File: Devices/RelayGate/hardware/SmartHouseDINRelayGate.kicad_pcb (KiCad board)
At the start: 2 copper layers, 31 x 82 mm, 14 parts, among them P1 CONN_UPDOWN_ONOFF_PWR_GND, P2 CONN_IN_DOWN_UP, Q1 Q_NPN_EBC, Q2 Q_NPN_EBC, Q3 Q_NPN_BCE_DTC124, Q4 Q_NPN_BCE_DTC124, U2 RELAY_1C, U3 RELAY_1C

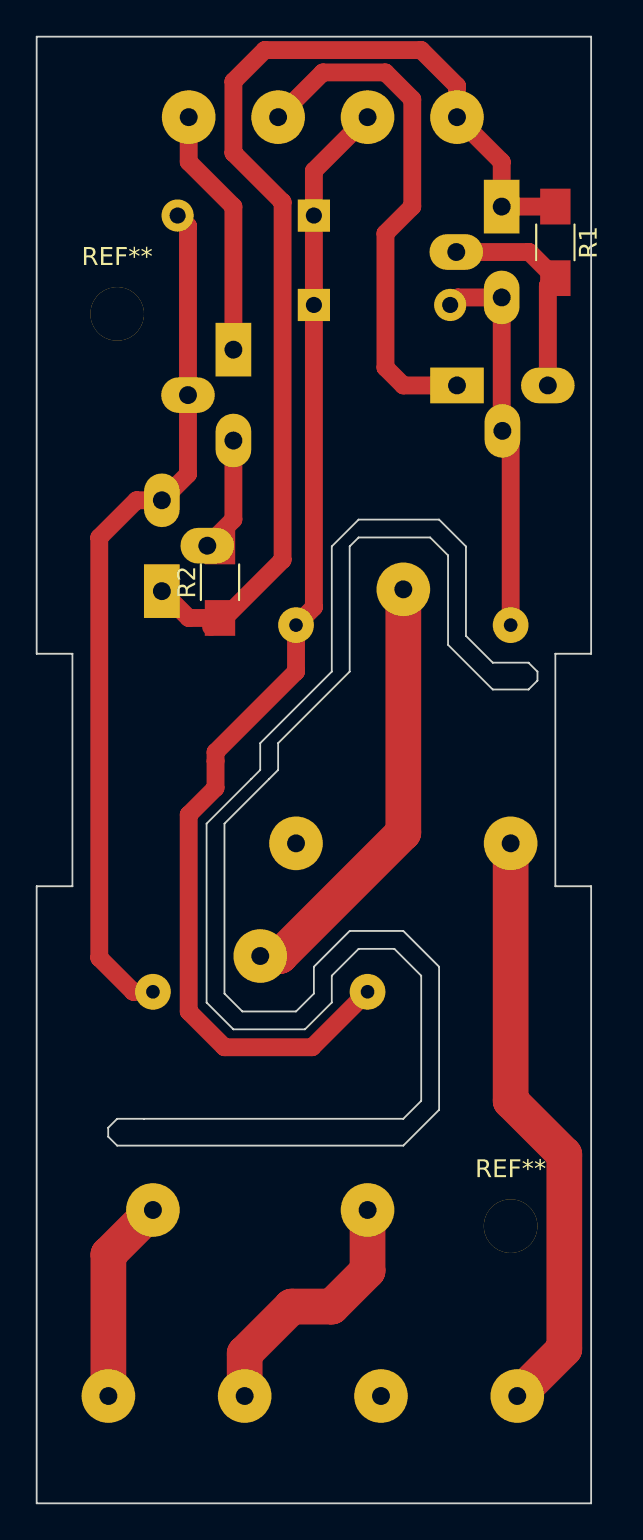
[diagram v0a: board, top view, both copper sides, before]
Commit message: -Devices updates
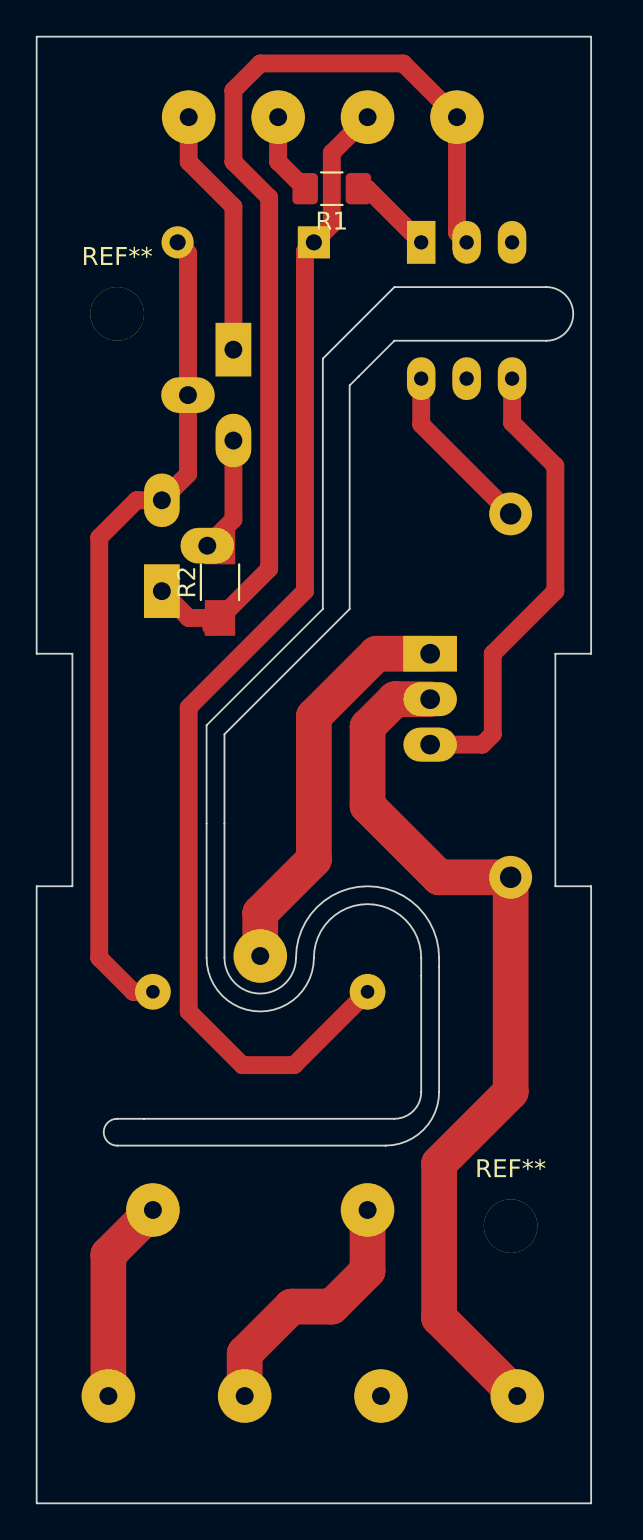
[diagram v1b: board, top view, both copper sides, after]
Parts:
- removed D1: D, Diodes_ThroughHole:D_A-405_P7.62mm_Horizontal
- removed Q3: Q_NPN_BCE_DTC124, TO_SOT_Packages_THT:TO-92_Rugged
- removed U2: RELAY_1C, SmartHouseLib:RELAY_TRU_1C
- added R3: R, Resistor_THT:R_Axial_DIN0414_L11.9mm_D4.5mm_P20.32mm_Horizontal, B.Cu at (275.0, 97.5)
- added U1: MOC3020M, Package_DIP:DIP-6_W7.62mm_LongPads, B.Cu at (270.0, 62.0)
- Q1: value Q_NPN_EBC -> BTA16-600B; footprint TO_SOT_Packages_THT:TO-92_Rugged -> Package_TO_SOT_THT:TO-220-3_Vertical
- R1: value R4K7 -> R; footprint Resistors_SMD:R_1206_HandSoldering -> Resistor_SMD:R_1206_3216Metric_Pad1.42x1.75mm_HandSolder
- moved Q1 25.3 mm to (270.5, 85.0)
- moved R1 12.9 mm to (265.0, 59.0), turned to 180 degrees
- moved D2 1.50 mm to (264.0, 62.0)
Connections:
- Q1 pad 1: Net-(P1-Pad4) -> Net-(Q1-Pad1)
- Q1 pad 2: Net-(Q1-Pad2) -> Net-(P2-Pad4)
- R1 pad 1: Net-(P1-Pad4) -> Net-(R1-Pad1)
- R1 pad 2: Net-(Q1-Pad2) -> Net-(P1-Pad2)
- U3 pad 3: Net-(U2-Pad3) -> Net-(Q1-Pad1)
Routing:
- net Net-(P1-Pad2): track 29.2 -> 4.63 mm
- net Net-(U2-Pad3): track 24.5 -> 0.00 mm
- net Net-(Q1-Pad1): track 0.00 -> 22.6 mm
- net Net-(P2-Pad4): track 33.2 -> 50.7 mm
- net Net-(Q1-Pad2): track 12.3 -> 0.00 mm
- net Net-(R3-Pad2): track 0.00 -> 9.63 mm
- net Net-(R1-Pad1): track 0.00 -> 4.76 mm
- net Net-(P1-Pad4): track 62.2 -> 57.6 mm
- net Net-(Q1-Pad3): track 21.6 -> 26.1 mm
- net Net-(D2-Pad2): track 48.4 -> 46.9 mm
- net Net-(D2-Pad1): track 66.4 -> 67.2 mm
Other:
- outline, holes or cut-outs redrawn
- board text added: "ASNP Relay Gate 3.0"
- board text removed: "ASNP Relay Gate 2.0"
